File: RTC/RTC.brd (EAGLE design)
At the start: 25.4 x 25.4 mm, 8 parts, among them IC1 DS3231/SO

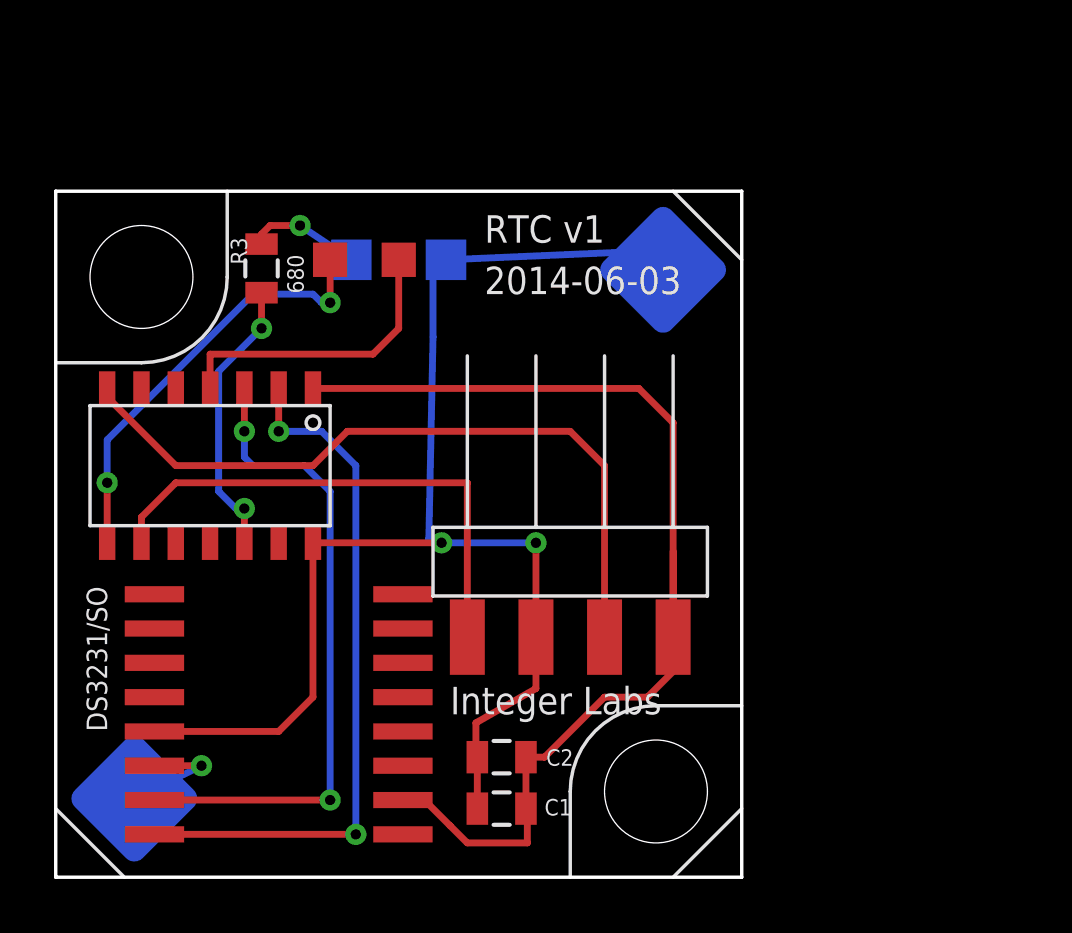
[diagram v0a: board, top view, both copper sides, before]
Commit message: Latest version of schematics and boards
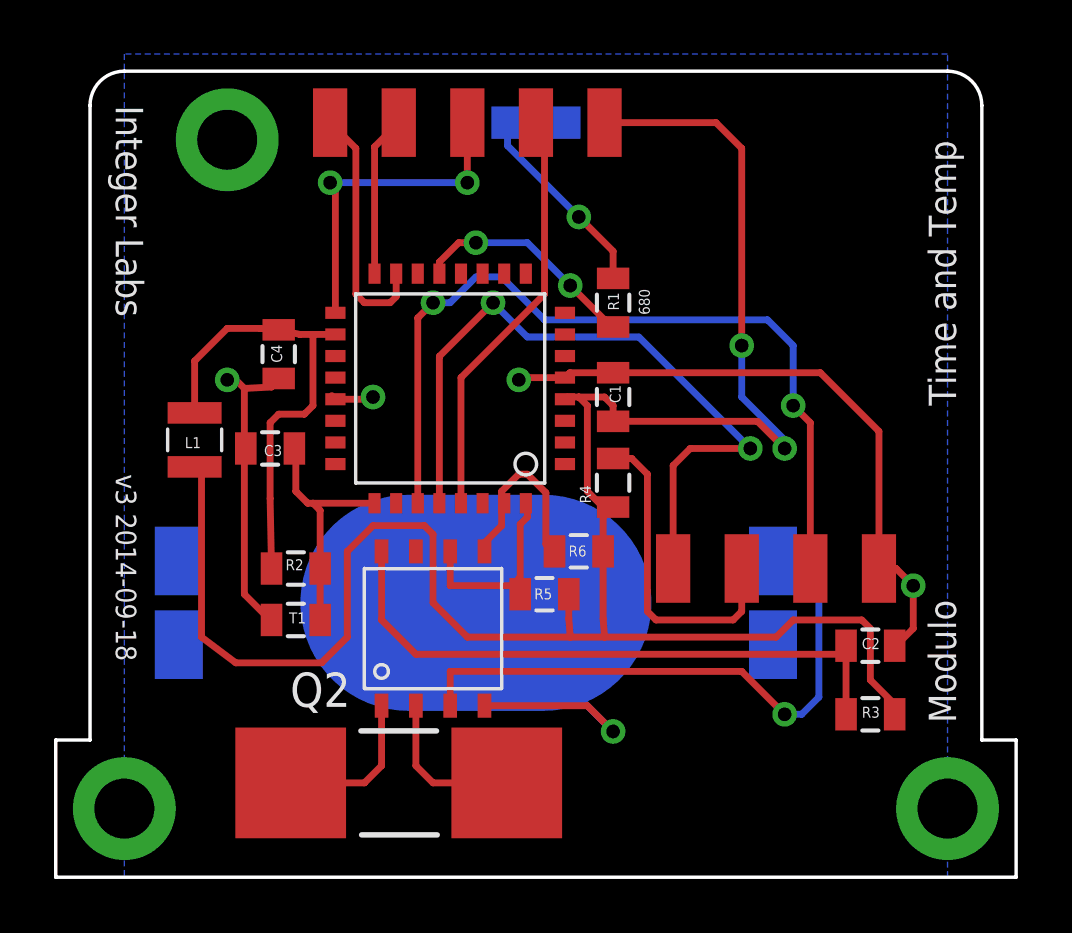
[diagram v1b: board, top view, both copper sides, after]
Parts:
- removed IC1: DS3231/SO, adafruit:SO16W
- removed LED: blue, led:CHIPLED_1206
- removed U$3: TINY841, IntegerLabs:SOIC14
- added BAT1: 20mm coincell, SparkFun-Electromechanical:BATTCON_20MM_4LEGS
- added C3: (no value), SparkFun-Capacitors:0805
- added C4: .47uF, SparkFun-Capacitors:0805
- added L1: 1mH, SparkFun-Passives:1007
- added LED1: (no value), adafruit:CHIP-LED0805
- added Q2: MC-405, crystal:MC-405
- added R1: 680, SparkFun-Passives:0805
- added R2: 10k, SparkFun-Passives:0805
- added R4: 1, SparkFun-Resistors:0805
- added R5, R6: 2k, SparkFun-Resistors:0805
- added T1: therm, SparkFun-Passives:0805
- added U$1: ATTINY48/88-TQFP, IntegerLabs:TQFP-32
- C1: value 0.1uF -> .47uF
- C2: value 10uF -> 2.2uF; device SparkFun-Capacitors:0805 -> SparkFun-Passives:0805
- R3: value 680 -> 1k
- U$2: value BATTERY -> PCF8523; device IntegerLabs:BU1632 -> IntegerLabs:SOIC-8
- U$4: value FOOTPRINT -> FOOTPRINTFOOTPRINT-2; device IntegerLabs:FOOTPRINT -> IntegerLabs:FOOTPRINT2
- moved R3 27.9 mm to (30.2, 6.03), turned to 0 degrees
- moved C1 15.8 mm to (20.6, 17.8), turned to 270 degrees
- moved C2 14.3 mm to (30.2, 8.57)
- moved U$4 10.2 mm to (35.6, 0.00)
- moved U$2 3.24 mm to (13.3, 9.53), flipped to the top, turned to 0 degrees
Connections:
- removed net DATA: U$3.11
- removed net SCL/SCK: U$3.9, U$4.P$4
- removed net SDA/MOSI: U$3.7, U$4.P$2
- new net AVCC: C4.2, L1.1, R2.1, U$1.18
- new net MOSI: U$1.15, U$4.PROG4
- new net N$7: Q2.1, U$2.1
- new net N$8: Q2.2, U$2.2
- new net RTC_CLKOUT: U$2.7
- new net RTC_SCL: R5.1, U$1.32, U$2.6
- new net RTC_SDA: R6.1, U$1.31, U$2.5
- new net SCK: U$1.17, U$4.PROG2
- new net SCL: U$1.28, U$4.BUS3
- new net SDA: U$1.27, U$4.BUS1
- new net THERM: C3.1, R2.2, T1.2, U$1.25
- net GND: now also BAT1.2, C2.2, C3.2, C4.1, LED1.C, T1.1, U$1.21, U$1.5, U$2.4, U$4.BUS0; no longer C2.1, IC1.13, LED.C, U$2.-, U$3.14, U$4.P$3
- net LED: now also R1.2, U$1.13; no longer R3.2, U$3.12
- net MISO: now also U$1.16, U$4.PROG3; no longer U$3.8, U$4.MISO
- net N$2: now also R4.2, U$4.BUS2; no longer IC1.16, U$3.2
- net N$3: now also C2.1, R3.1, U$2.8; no longer IC1.15, U$3.3
- net N$5: now also LED1.A, R1.1; no longer LED.A, R3.1
- net RESET: now also U$1.29, U$4.PROG1; no longer U$3.4, U$4.RESET
- net VBAT: now also BAT1.1, U$2.3; no longer IC1.14, U$2.+
- net VCC: now also L1.2, R3.2, R4.1, R5.2, R6.2, U$1.4, U$4.PROG0; no longer C2.2, IC1.2, U$3.1, U$4.P$1
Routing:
- net VCC: track 41.5 -> 80.5 mm, vias 0 -> 2
- net SDA: track 0.00 -> 31.0 mm, vias 0 -> 2
- net SDA/MOSI: track 27.2 -> 0.00 mm
- net SCL: track 0.00 -> 26.9 mm, vias 0 -> 2
- net SCL/SCK: track 19.6 -> 0.00 mm
- net VBAT: track 4.51 -> 22.4 mm
- net AVCC: track 0.00 -> 17.7 mm
- net N$2: track 26.1 -> 11.9 mm, vias 2 -> 0
- net SCK: track 0.00 -> 12.2 mm, vias 0 -> 2
- net MISO: track 16.0 -> 5.96 mm, vias 2 -> 0
- net MOSI: track 0.00 -> 9.31 mm
- net THERM: track 0.00 -> 9.14 mm
- net RTC_SCL: track 0.00 -> 8.35 mm
- net RTC_SDA: track 0.00 -> 7.08 mm
- net N$7: track 0.00 -> 5.85 mm
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- added copper zone on layer 16, net GND
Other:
- board size 25.4 x 25.4 mm -> 35.6 x 29.8 mm
- board text added: "Modulo"
- board text added: "Time and Temp"
- board text added: "v3 2014-09-18"
- board text removed: "2014-06-03"
- board text removed: "RTC v1"
